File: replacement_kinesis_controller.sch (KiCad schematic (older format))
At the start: 50 parts

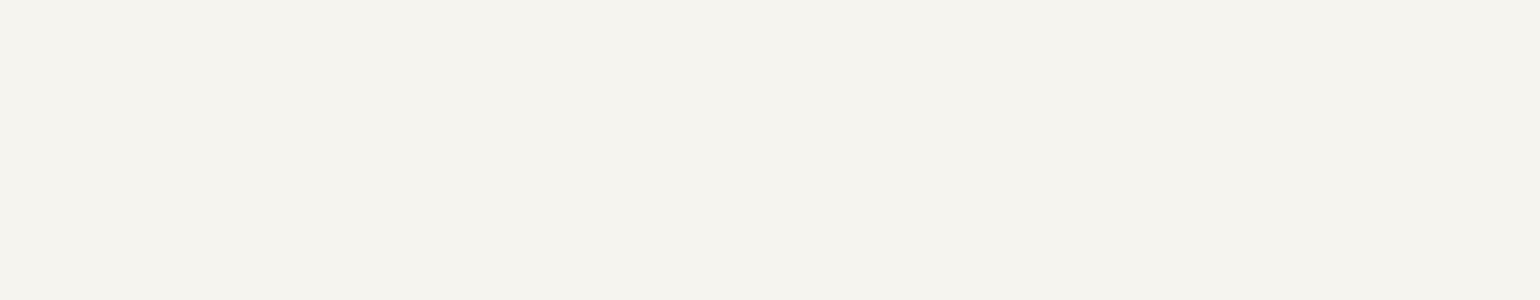
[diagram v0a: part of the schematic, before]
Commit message: More stuff, including LEDs
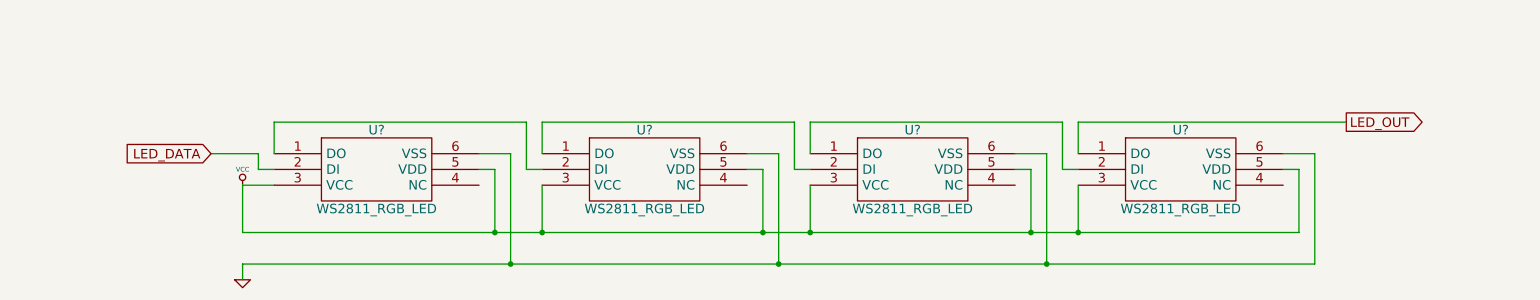
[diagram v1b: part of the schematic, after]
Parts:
- added U? (x4): WS2811_RGB_LED, symbol WS2811_RGB_LED
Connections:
- net GND: now also U?.6 (VSS), U?.6 (VSS), U?.6 (VSS), U?.6 (VSS)
- net VCC: now also U?.3 (VCC), U?.3 (VCC), U?.3 (VCC), U?.3 (VCC), U?.5 (VDD), U?.5 (VDD), U?.5 (VDD), U?.5 (VDD)
- new net: U?.1 (DO), U?.2 (DI) (x3)
- new net LED_DATA: U?.2 (DI)
- new net LED_OUT: U?.1 (DO)
